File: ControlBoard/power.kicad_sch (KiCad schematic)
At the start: 29 parts, among them Q1 PMOS

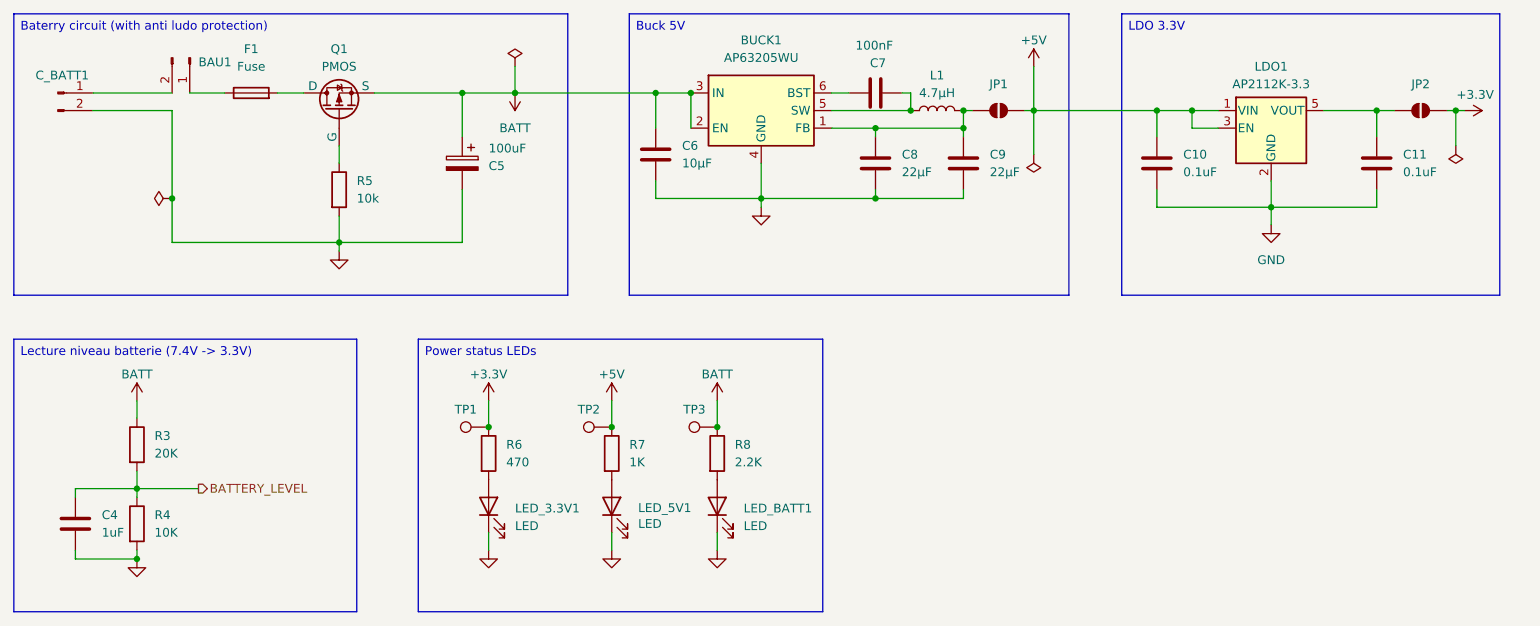
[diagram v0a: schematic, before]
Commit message: Feat: multiplex power over usb + add gitignore
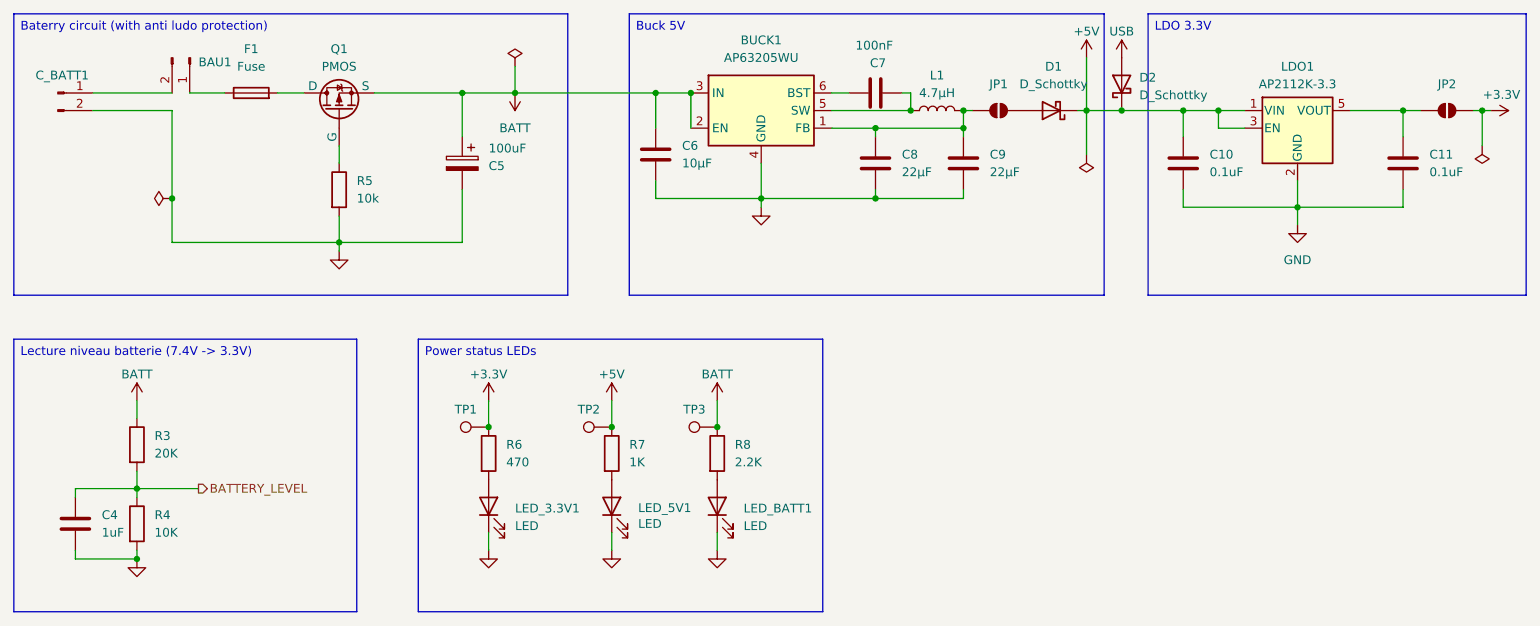
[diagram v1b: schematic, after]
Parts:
- added D1, D2: D_Schottky, Diode_SMD:D_0603_1608Metric, symbol Device:D_Schottky
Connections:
- net +5V: now also D1.1 (K), D2.1 (K); no longer JP1.2 (B)
- new net: D1.2 (A), JP1.2 (B)
- new net USB: D2.2 (A)
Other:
- moved on the sheet: C10, C11, JP2, LDO1
